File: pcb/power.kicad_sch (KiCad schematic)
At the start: 9 parts

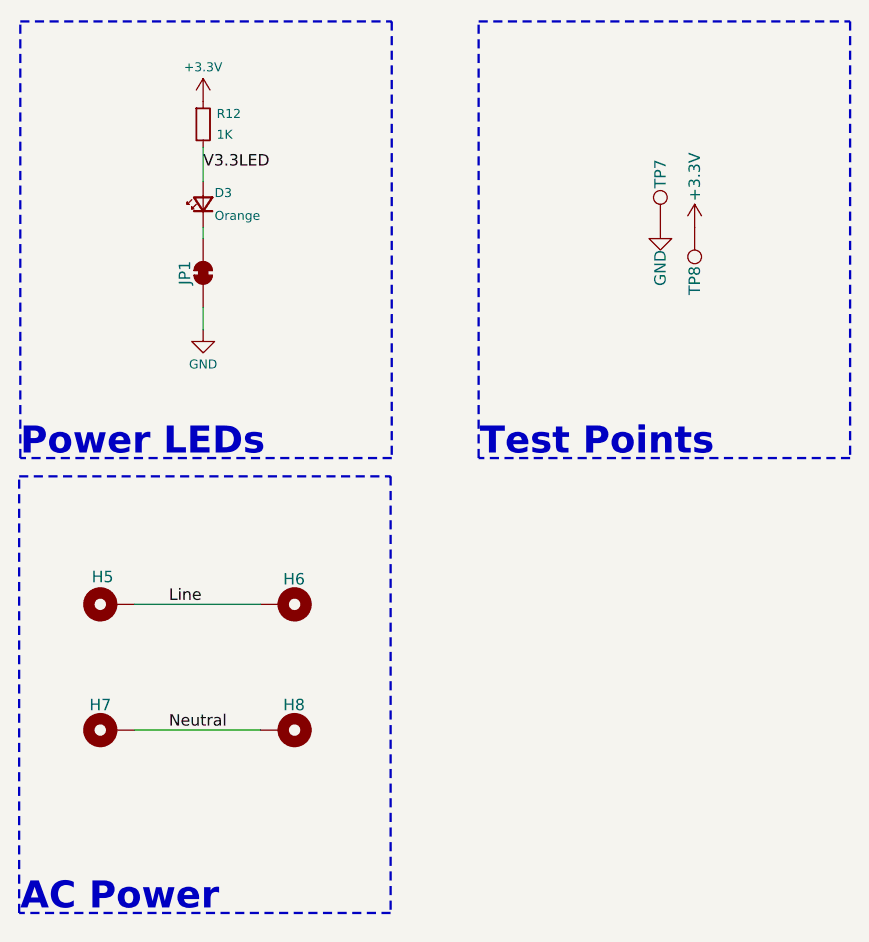
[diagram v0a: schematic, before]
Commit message: Redesign with MCU
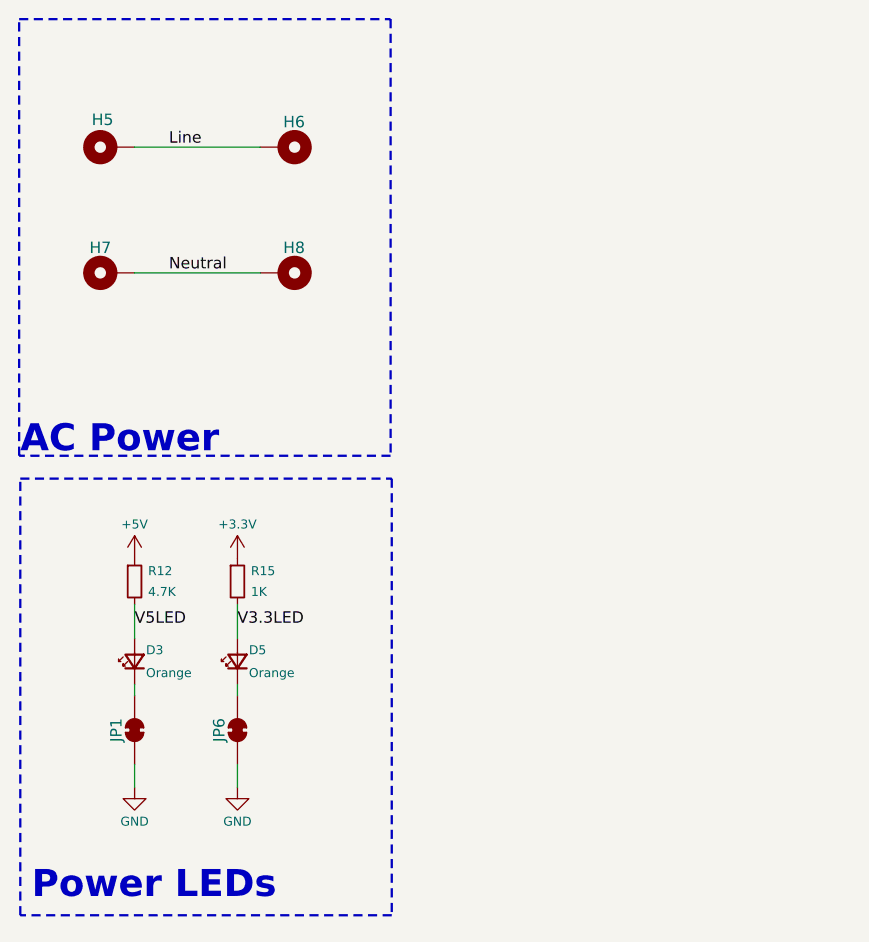
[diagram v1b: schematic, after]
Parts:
- removed TP7, TP8: ~, CRGM Mechanical:TestPoint_Pad_D1.0mm, symbol Connector:TestPoint
- added D3: Orange, CRGM Passive:LED_0603_1608Metric, symbol Device:LED_Small
- added JP1: ~, CRGM Connector:SolderJumper-2_P1.3mm_Bridged_RoundedPad1.0x1.5mm, symbol Jumper:SolderJumper_2_Bridged
- added R15: 1K, CRGM Passive:R_0603_1608Metric, symbol Device:R_Small
- D5: renamed from D3; footprint CRG Makes:LED_0603_1608Metric -> CRGM Passive:LED_0603_1608Metric
- R12: value 1K -> 4.7K; Digikey 541-3991-2-ND -> 541-3993-2-ND; LCSC C2907113 -> C2907166; MPN FRC0603J102 TS -> FRC0603J472 TS; Mouser 71-CRCW06031K00JNEAC -> 71-CRCW06034K70JNEAC; Tolerance 5% -> (none)
- renumbered JP1 to JP6
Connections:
- net +3.3V: now also R15.1; no longer R12.1
- net GND: now also JP1.1 (A)
- net V3.3LED: now also R15.2; no longer R12.2
- new net: D3.1 (K), JP1.2 (B)
- new net +5V: R12.1
- new net V5LED: D3.2 (A), R12.2
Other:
- note removed: "Test Points"
- moved on the sheet: D5, H5, H6, H7, H8, JP6
